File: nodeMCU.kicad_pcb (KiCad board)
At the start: 2 copper layers, 25.4 x 48.3 mm, 38 parts, among them J1 USB_B_Micro, J2 Conn_01x15, J3 Conn_01x15, Q1 S8050, Q2 S8050, SW1 RESET, SW2 FLASH, U1 AP1117-33, U2 CP2102N-A01-GQFN28, U3 ESP-12E

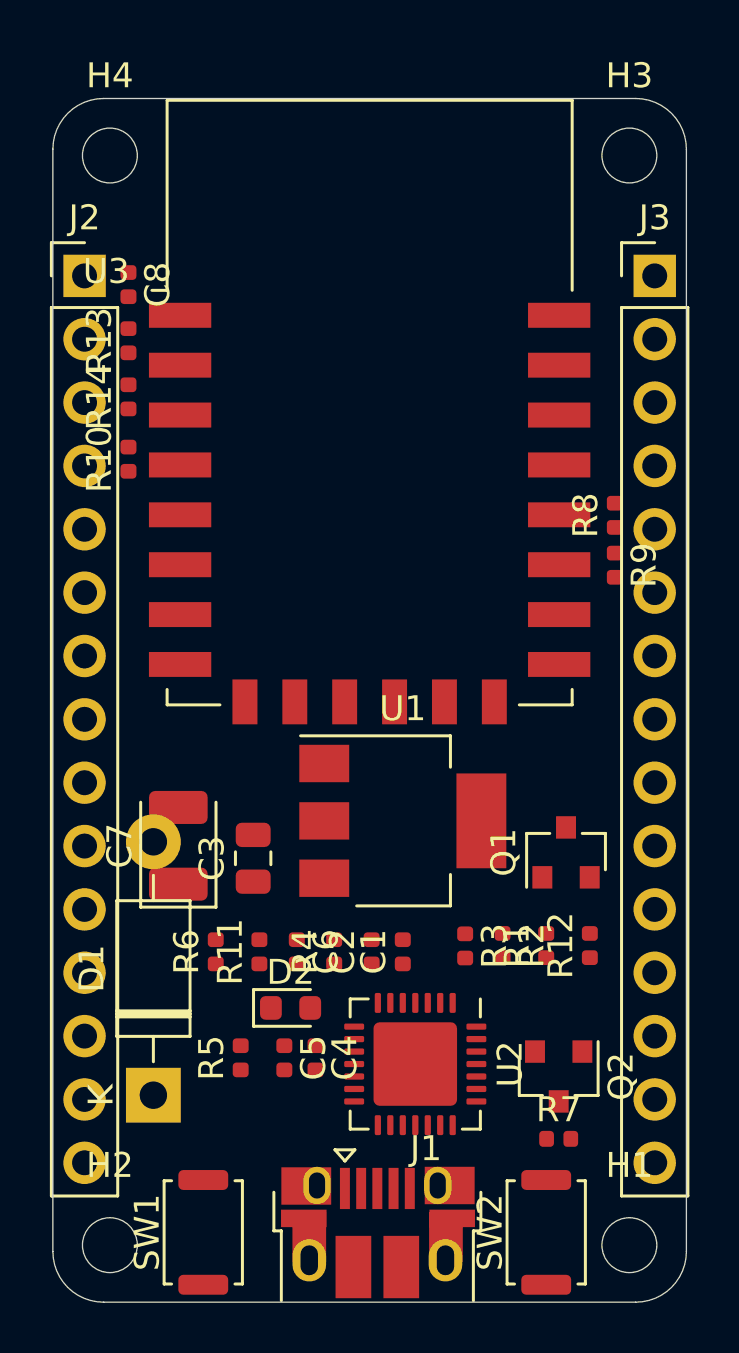
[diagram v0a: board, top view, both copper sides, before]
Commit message: Comienzo el ruteo
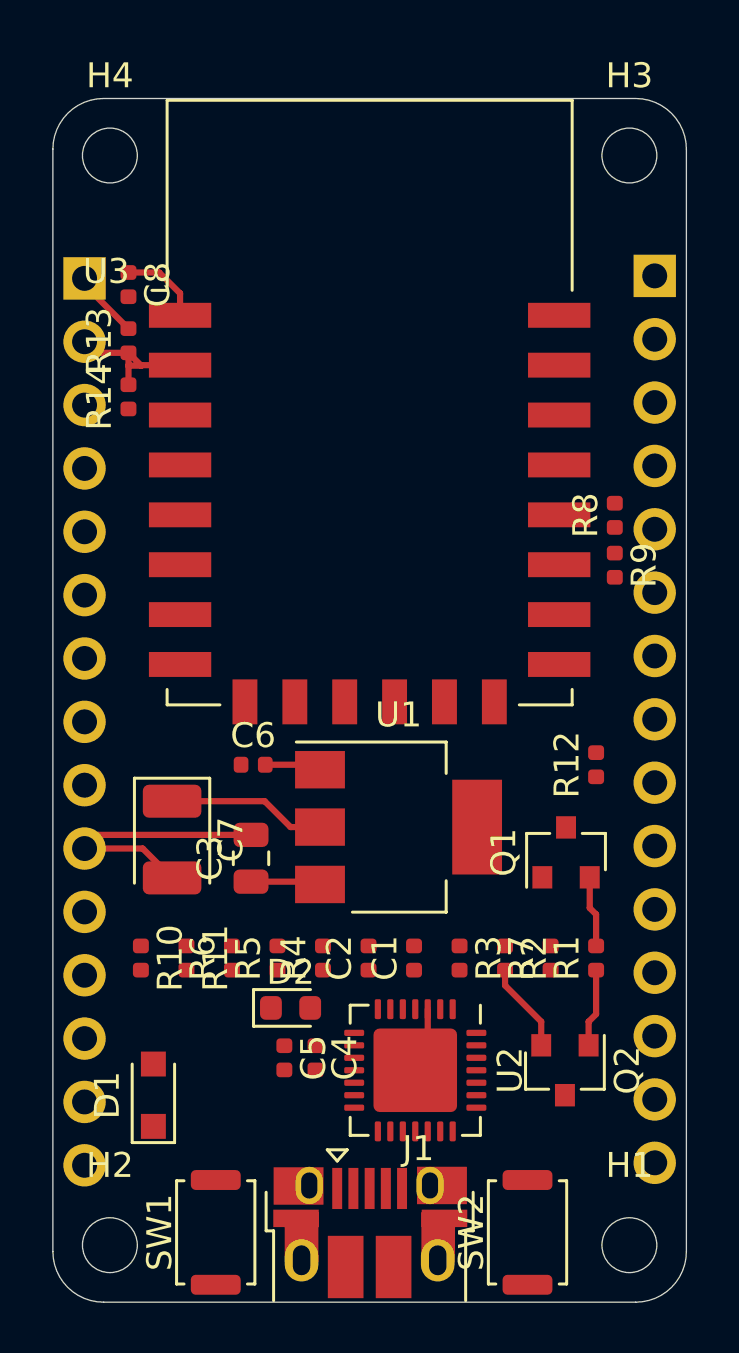
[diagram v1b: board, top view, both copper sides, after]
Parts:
- D1: footprint Diode_THT:D_DO-41_SOD81_P10.16mm_Horizontal -> Diode_SMD:D_SOD-323_HandSoldering
- J2, J3: moved to B.Cu
- moved R10 20.0 mm to (176.2, 84.5), turned to 270 degrees
- moved C6 7.70 mm to (180.8, 76.8), turned to 0 degrees
- moved R7 7.26 mm to (192.7, 84.5), turned to 90 degrees
- moved R12 7.25 mm to (194.5, 76.8)
- moved R5 4.26 mm to (181.7, 84.5)
- moved R11 2.94 mm to (178.1, 84.5), turned to 270 degrees
- moved R1 2.06 mm to (194.5, 84.5)
- moved SW2 0.75 mm to (191.8, 95.5)
- moved R6 0.70 mm to (179.9, 84.5)
- moved R3 0.53 mm to (189.0, 84.5)
- moved C1 0.51 mm to (187.2, 84.5)
- moved R4 0.51 mm to (183.6, 84.5)
- moved R2 0.51 mm to (190.8, 84.5)
- moved SW1 0.50 mm to (179.2, 95.5)
- moved C7 0.35 mm to (177.5, 79.8), turned to 270 degrees
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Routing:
- net GND: track 0.00 -> 15.8 mm
- net +3V3: track 0.00 -> 6.36 mm
- net /ADC: track 0.00 -> 6.03 mm
- net Net-(Q2-Pad2): track 0.00 -> 3.62 mm
- net /nRST: track 0.00 -> 3.30 mm
- net /nRTS_CP: track 0.00 -> 3.14 mm
- net Net-(Q1-Pad2): track 0.00 -> 2.86 mm
- net +5V: track 0.00 -> 2.81 mm
- net /ADC_EX: track 0.00 -> 2.74 mm
